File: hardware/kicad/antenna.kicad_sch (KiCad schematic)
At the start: 11 parts, among them J6 BWIPX-1-001E, J7 BWIPX-1-001E

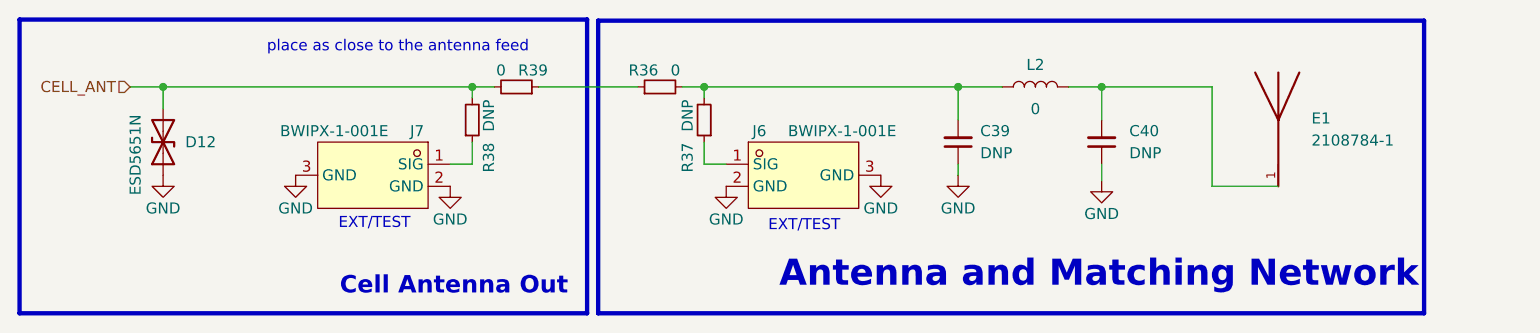
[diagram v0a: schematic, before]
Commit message: update
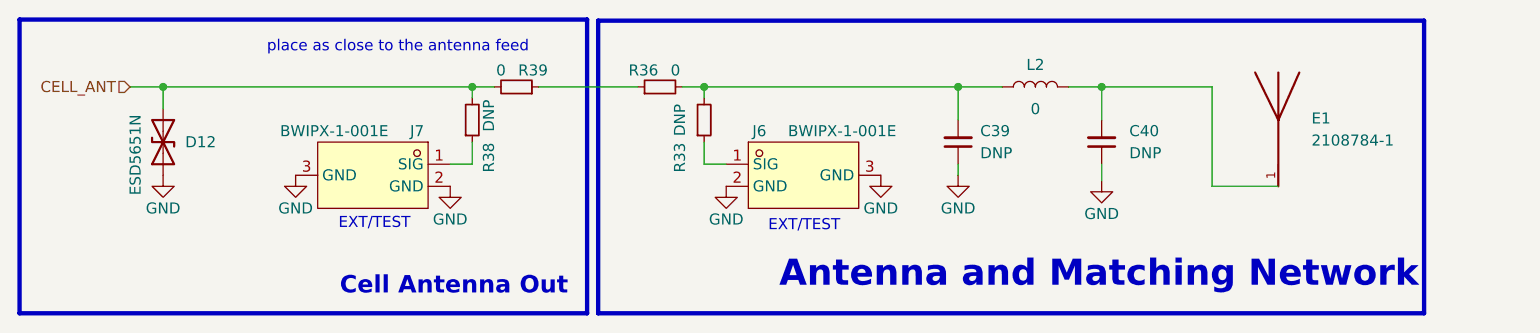
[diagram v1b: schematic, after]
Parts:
- removed R37: DNP, Resistor_SMD:R_0402_1005Metric, symbol Device:R_Small
- added R33: DNP, Resistor_SMD:R_0402_1005Metric, symbol Device:R_Small
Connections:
- net at C39.2, L2.1, R36.2: now also R33.2
- net at J6.1 (SIG): now also R33.1
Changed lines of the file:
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@@
-	)
-	(symbol
-		(lib_id "Device:R_Small")
-		(at 153.67 93.98 180)
-		(unit 1)
-		(exclude_from_sim no)
-		(in_bom yes)
-		(on_board yes)
-		(dnp no)
-		(property "Reference" "R37"
-			(at 151.765 98.298 90)
-			(effects
-				(font
-					(size 1.27 1.27)
-				)
-			)
-		)
-		(property "Value" "DNP"
-			(at 151.765 93.472 90)
-			(effects
-				(font
-					(size 1.27 1.27)
-				)
-			)
-		)
-		(property "Footprint" "Resistor_SMD:R_0402_1005Metric"
-			(at 153.67 93.98 0)
-			(effects
-				(font
-					(size 1.27 1.27)
-				)
-				(hide yes)
-			)
-		)
-		(property "Datasheet" ""
-			(at 153.67 93.98 0)
-			(effects
-				(font
-					(size 1.27 1.27)
-				)
-				(hide yes)
-			)
-		)
-		(property "Description" ""
-			(at 153.67 93.98 0)
-			(effects
-				(font
-					(size 1.27 1.27)
-				)
-				(hide yes)
-			)
-		)
-		(property "Manufacturer" ""
-			(at 153.67 93.98 0)
-			(effects
-				(font
-					(size 1.27 1.27)
-				)
-				(hide yes)
-			)
-		)
-		(property "Manufacturer Part Number" ""
-			(at 153.67 93.98 0)
-			(effects
-				(font
-					(size 1.27 1.27)
-				)
-				(hide yes)
-			)
-		)
-		(property "Distributor" ""
-			(at 153.67 93.98 0)
-			(effects
-				(font
-					(size 1.27 1.27)
-				)
-				(hide yes)
-			)
-		)
-		(property "Distributor Part Number" ""
-			(at 153.67 93.98 0)
-			(effects
-				(font
-					(size 1.27 1.27)
-				)
-				(hide yes)
-			)
-		)
-		(property "Distributor Link" ""
-			(at 153.67 93.98 0)
-			(effects
-				(font
-					(size 1.27 1.27)
-				)
-				(hide yes)
-			)
-		)
-		(property "Id" ""
-			(at 153.67 93.98 0)
-			(effects
-				(font
-					(size 1.27 1.27)
-				)
-				(hide yes)
-			)
-		)
-		(property "Manufacture" ""
-			(at 153.67 93.98 0)
-			(effects
-				(font
-					(size 1.27 1.27)
-				)
-				(hide yes)
-			)
-		)
-		(property "Manufacture Part Number" ""
-			(at 153.67 93.98 0)
-			(effects
-				(font
-					(size 1.27 1.27)
-				)
-				(hide yes)
-			)
-		)
-		(property "Type" ""
-			(at 153.67 93.98 0)
-			(effects
-				(font
-					(size 1.27 1.27)
-				)
-				(hide yes)
-			)
-		)
-		(pin "1"
-		)
-		(pin "2"
-		)
-		(instances
-			(project "bwlc1a"
-				(path "/388039b1-99cc-430f-bd4a-010573fde798/ca79f09e-abdb-462a-9aab-98f2e37e5b23"
-					(reference "R37")
-					(unit 1)
-				)
-			)
-		)
 	)
 	(symbol
@@
 					(unit 1)
 				)
+			)
+		)
+	)
+	(symbol
+		(lib_id "Device:R_Small")
+		(at 153.67 93.98 0)
+		(mirror x)
+		(unit 1)
+		(exclude_from_sim no)
+		(in_bom yes)
+		(on_board yes)
+		(dnp no)
+		(property "Reference" "R33"
+			(at 150.876 98.298 90)
+			(effects
+				(font
+					(size 1.27 1.27)
+				)
+			)
+		)
+		(property "Value" "DNP"
+			(at 150.876 93.98 90)
+			(effects
+				(font
+					(size 1.27 1.27)
+				)
+			)
+		)
+		(property "Footprint" "Resistor_SMD:R_0402_1005Metric"
+			(at 153.67 93.98 0)
+			(effects
+				(font
+					(size 1.27 1.27)
+				)
+				(hide yes)
+			)
+		)
+		(property "Datasheet" ""
+			(at 153.67 93.98 0)
+			(effects
+				(font
+					(size 1.27 1.27)
+				)
+				(hide yes)
+			)
+		)
+		(property "Description" ""
+			(at 153.67 93.98 0)
+			(effects
+				(font
+					(size 1.27 1.27)
+				)
+				(hide yes)
+			)
+		)
+		(property "Manufacturer" ""
+			(at 153.67 93.98 0)
+			(effects
+				(font
+					(size 1.27 1.27)
+				)
+				(hide yes)
+			)
+		)
+		(property "Manufacturer Part Number" ""
+			(at 153.67 93.98 0)
+			(effects
+				(font
+					(size 1.27 1.27)
+				)
+				(hide yes)
+			)
+		)
+		(property "Distributor" ""
+			(at 153.67 93.98 0)
+			(effects
+				(font
+					(size 1.27 1.27)
+				)
+				(hide yes)
+			)
+		)
+		(property "Distributor Part Number" ""
+			(at 153.67 93.98 0)
+			(effects
+				(font
+					(size 1.27 1.27)
+				)
+				(hide yes)
+			)
+		)
+		(property "Distributor Link" ""
+			(at 153.67 93.98 0)
+			(effects
+				(font
+					(size 1.27 1.27)
+				)
+				(hide yes)
+			)
+		)
+		(property "Id" ""
+			(at 153.67 93.98 0)
+			(effects
+				(font
+					(size 1.27 1.27)
+				)
+				(hide yes)
+			)
+		)
+		(property "Manufacture" ""
+			(at 153.67 93.98 0)
+			(effects
+				(font
+					(size 1.27 1.27)
+				)
+				(hide yes)
+			)
+		)
+		(property "Manufacture Part Number" ""
+			(at 153.67 93.98 0)
+			(effects
+				(font
+					(size 1.27 1.27)
+				)
+				(hide yes)
+			)
+		)
+		(property "Type" ""
+			(at 153.67 93.98 0)
+			(effects
+				(font
+					(size 1.27 1.27)
+				)
+				(hide yes)
+			)
+		)
+		(pin "1"
+		)
+		(pin "2"
+		)
+		(instances
+			(project "bwlc1a"
+				(path "/388039b1-99cc-430f-bd4a-010573fde798/ca79f09e-abdb-462a-9aab-98f2e37e5b23"
+					(reference "R33")
+					(unit 1)
+				)
